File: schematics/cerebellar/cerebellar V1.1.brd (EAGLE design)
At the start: 95.9 x 90.5 mm, 68 parts, among them CON1 ODRV2, CON2 ODRV1, CON3 ODRV3, CON4 ODRV4, CON5 ODRV5, CON6 ODRV6, IC3 LTC7001, P1 Foot1, P11 Foot2, P12 Foot3, P13 Foot4, P14 IMU, P15 ON, P16 MAG, P17 SPI2, P2 ODrive1, P3 SPI1, P4 LED, P5 ODrive2, P6 ODrive3, P7 ODrive4, P8 ODrive5, P9 ODrive6, U2 INA226AIDGST

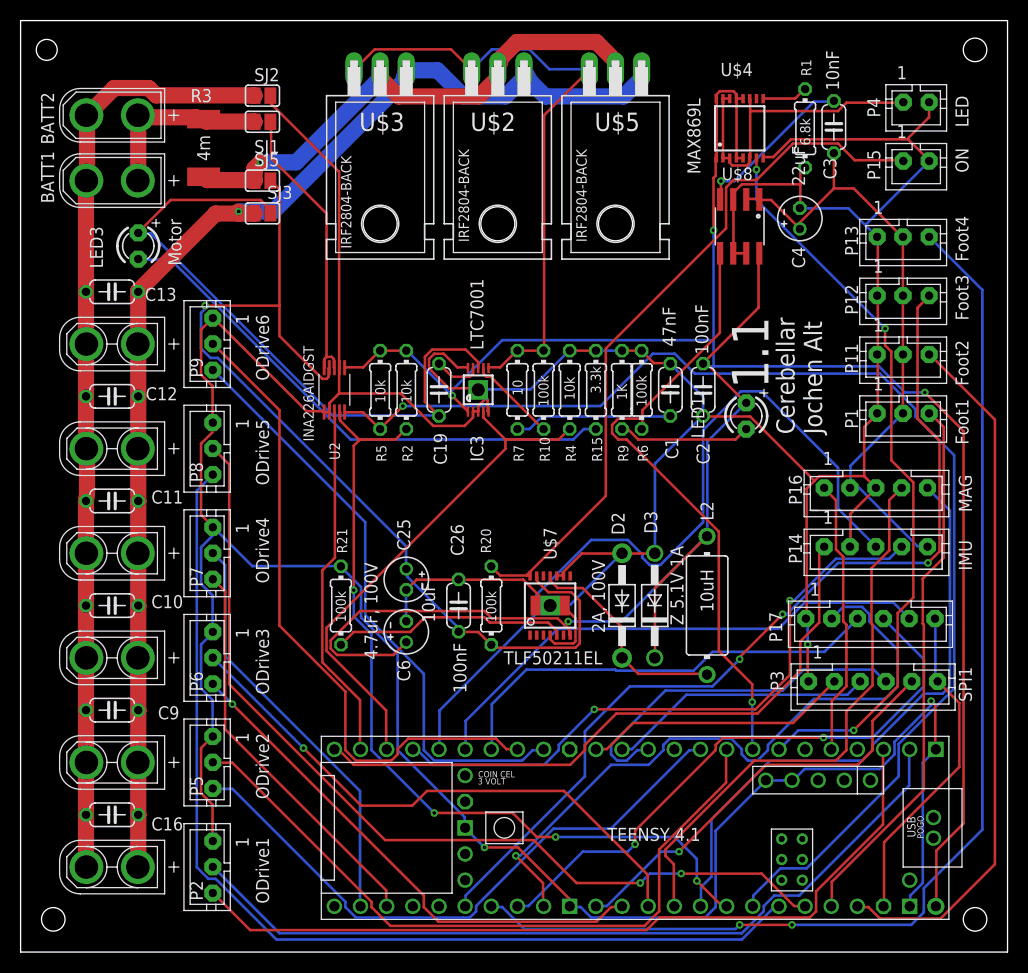
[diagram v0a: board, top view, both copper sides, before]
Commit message: started Raspi
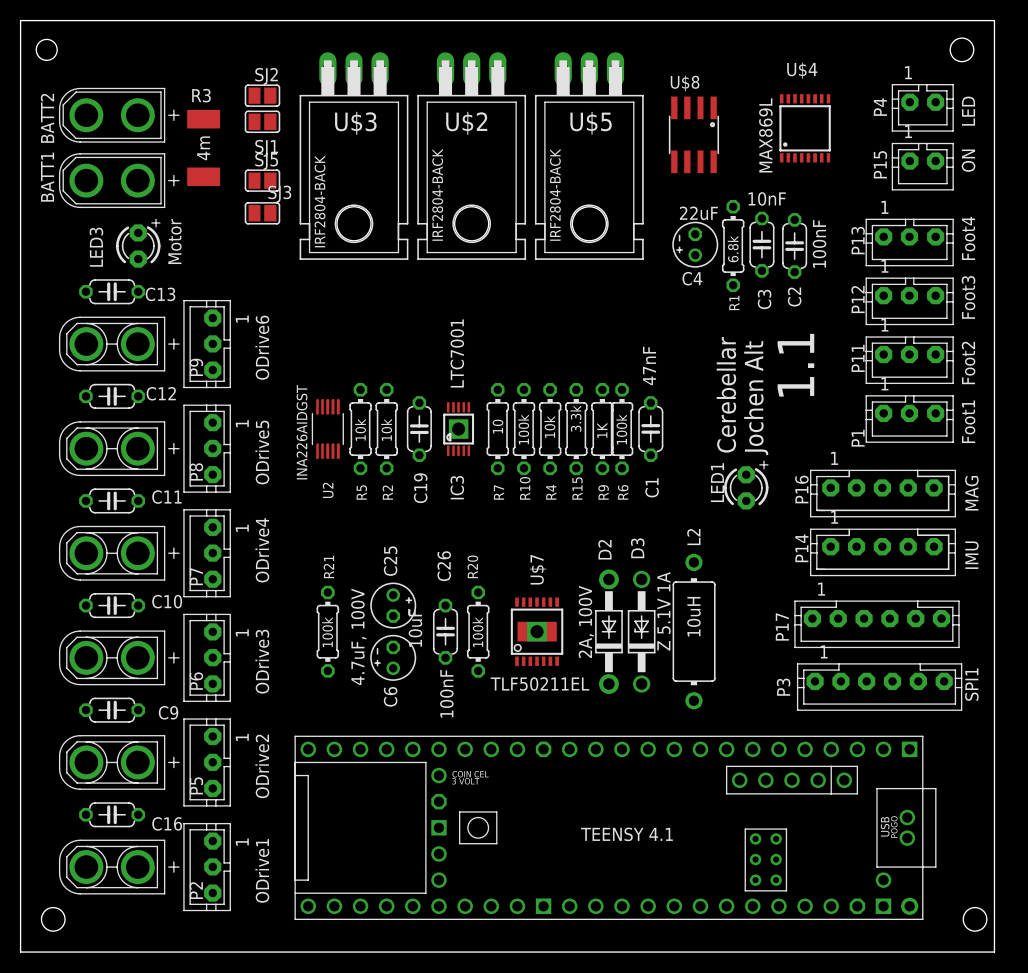
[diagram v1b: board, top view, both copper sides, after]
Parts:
- moved C2 16.6 mm to (68.8, 68.6)
- moved C3 13.4 mm to (65.7, 68.7)
- moved R1 13.4 mm to (62.9, 68.6)
- moved C4 10.5 mm to (59.2, 68.7)
- moved U$8 9.94 mm to (59.1, 79.4)
- moved LED1 6.98 mm to (64.1, 45.1)
- moved U$4 6.35 mm to (69.8, 80.0)
- moved C1 4.26 mm to (54.9, 50.8)
- moved C19 4.26 mm to (32.4, 50.8)
- moved IC3 4.26 mm to (36.2, 50.8)
- moved R10 4.26 mm to (42.5, 50.8)
- moved R15 4.26 mm to (47.6, 50.8)
- moved R4 4.26 mm to (45.1, 50.8)
- moved R6 4.26 mm to (52.1, 50.8)
- moved R9 4.26 mm to (50.2, 50.8)
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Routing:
- net GND: track 482.7 -> 0.00 mm, vias 3 -> 0
- net +5V: track 254.2 -> 0.00 mm, vias 4 -> 0
- net POWER+: track 121.5 -> 0.00 mm, vias 1 -> 0
- net N$17: track 120.8 -> 0.00 mm, vias 1 -> 0
- net SENS4: track 113.7 -> 0.00 mm, vias 2 -> 0
- net O5_TX: track 99.6 -> 0.00 mm
- net PMS+: track 95.0 -> 0.00 mm, vias 1 -> 0
- net BATT-: track 90.9 -> 0.00 mm
- net SENS3: track 89.8 -> 0.00 mm, vias 3 -> 0
- net O5_RX: track 89.2 -> 0.00 mm, vias 2 -> 0
- net N$22: track 81.6 -> 0.00 mm, vias 4 -> 0
- net O1_RX: track 80.1 -> 0.00 mm
- net O1_TX: track 79.3 -> 0.00 mm
- net TXD: track 76.2 -> 0.00 mm
- net LED_PWM: track 72.3 -> 0.00 mm, vias 3 -> 0
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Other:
- board size 95.9 x 90.5 mm -> 94.6 x 90.5 mm
